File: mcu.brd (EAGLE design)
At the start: 100 x 80 mm, 62 parts, among them IC1 MCP73831/OT, T1 SI7051-A20, U12 BQ297XY, U4 NRF52832, U7 CP2102N-A01-GQFN24, X1 LFXTAL069526, X6 32.768kHz

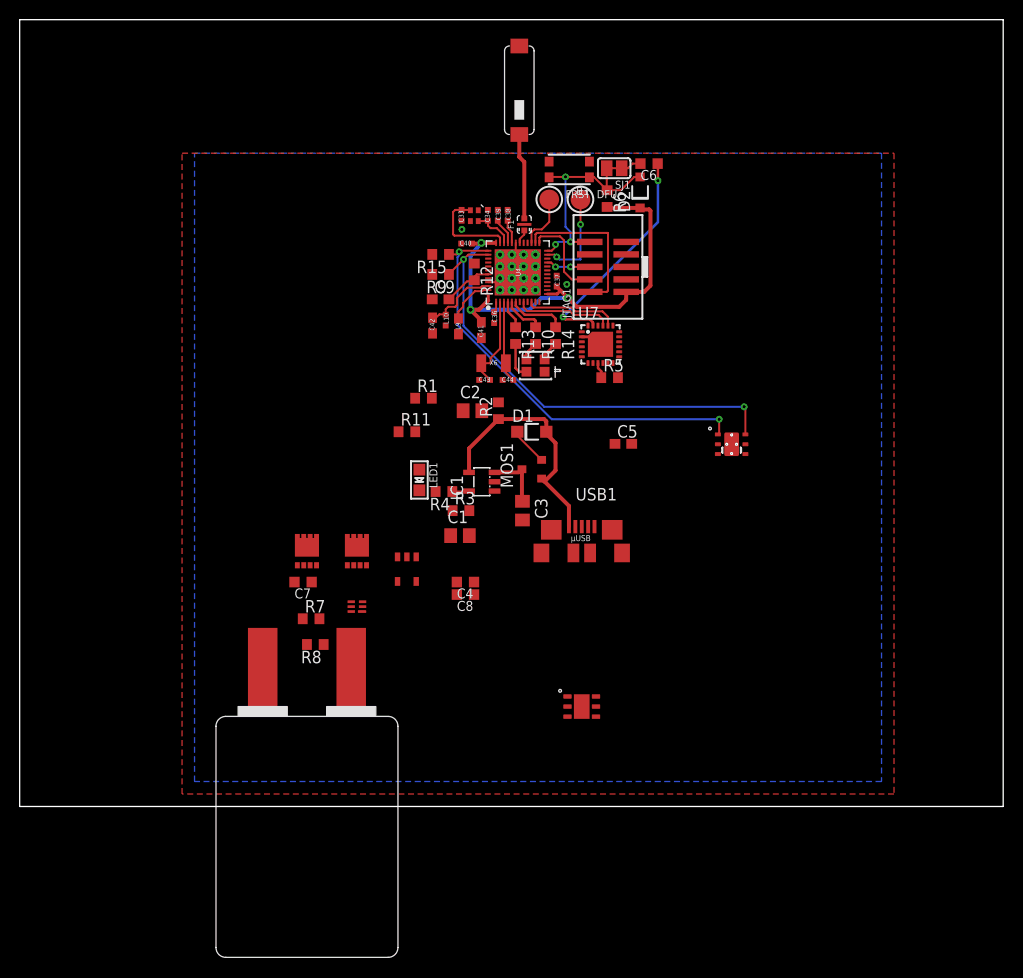
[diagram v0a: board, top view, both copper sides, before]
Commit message: UPD: finished wiring
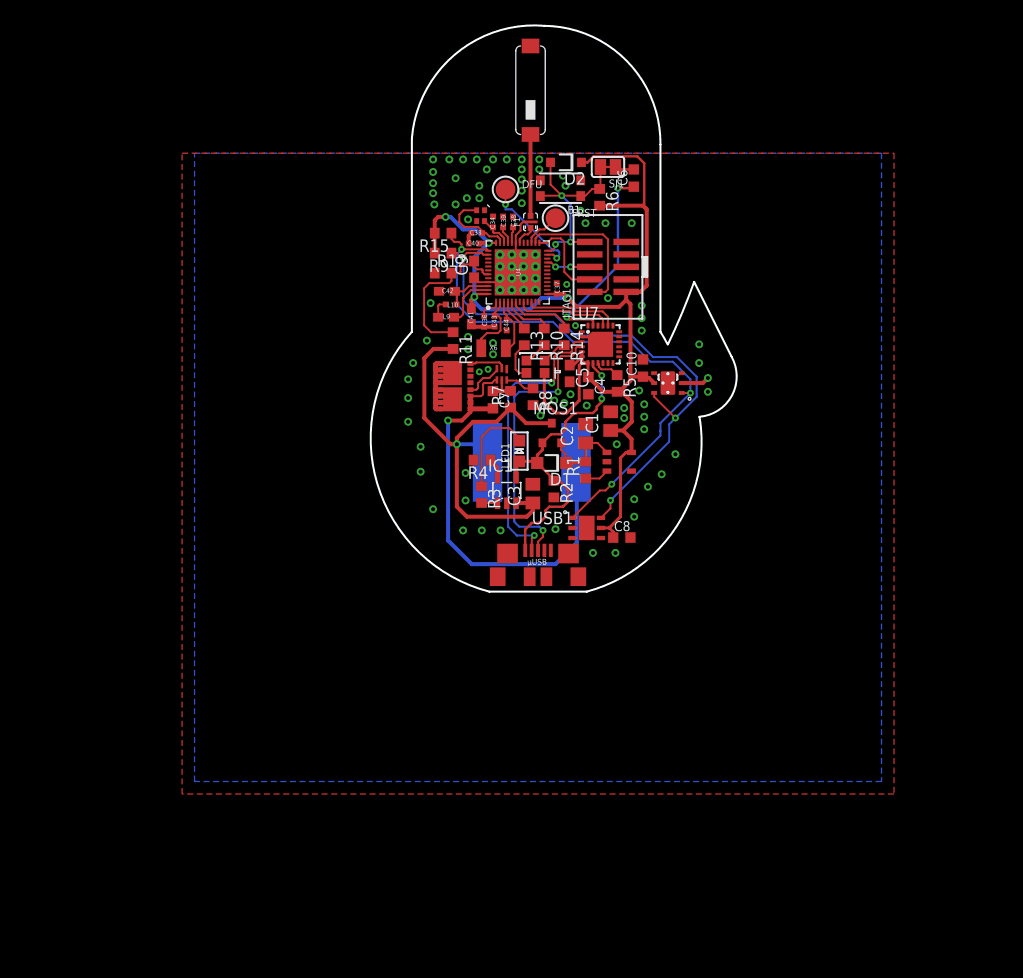
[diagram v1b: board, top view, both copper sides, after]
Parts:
- added C10: 0.1µF, rcl:C0603K
- moved U$14 36.8 mm to (52.1, 39.0), flipped to the bottom, turned to 180 degrees
- moved R8 33.5 mm to (52.2, 41.7), turned to 270 degrees
- moved R7 30.2 mm to (49.9, 41.4), turned to 90 degrees
- moved U12 27.8 mm to (49.0, 43.9), turned to 180 degrees
- moved C7 26.8 mm to (48.1, 41.4), turned to 270 degrees
- moved LDO1 24.2 mm to (61.0, 35.1), turned to 90 degrees
- moved C4 23.6 mm to (57.8, 42.8), turned to 270 degrees
- moved DSG 22.5 mm to (45.0, 41.4), turned to 90 degrees
- moved CHG 21.5 mm to (45.0, 44.1), turned to 90 degrees
- moved C1 19.2 mm to (60.1, 39.2), turned to 90 degrees
- moved T1 18.2 mm to (57.7, 28.3)
- moved R1 18.0 mm to (57.5, 34.2), turned to 90 degrees
- moved C8 16.9 mm to (61.2, 27.3), turned to 0 degrees
- moved C2 11.7 mm to (57.5, 37.9), turned to 90 degrees
- moved LED1 10.6 mm to (50.8, 36.1), turned to 0 degrees
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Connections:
- net GND: now also C10.2
- net V+: now also C10.1
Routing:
- net V+: track 50.0 -> 120.5 mm, vias 3 -> 4
- net N$16: track 0.00 -> 46.2 mm, vias 0 -> 1
- net VBAT: track 6.19 -> 47.9 mm, vias 0 -> 1
- net USBD+: track 0.00 -> 29.9 mm, vias 0 -> 2
- net USBD-: track 0.00 -> 29.4 mm, vias 0 -> 2
- net P0.25: track 43.8 -> 58.1 mm, vias 2 -> 3
- net N$11: track 0.00 -> 11.7 mm
- net P0.31: track 5.21 -> 16.5 mm
- net P0.26: track 46.4 -> 57.4 mm, vias 2 -> 3
- net GND: track 24.0 -> 34.8 mm, vias 2 -> 80
- net N$4: track 0.00 -> 9.91 mm
- net VUSB: track 24.6 -> 32.6 mm, vias 0 -> 2
- net N$2: track 3.89 -> 8.76 mm
- net N$12: track 0.00 -> 3.98 mm
- net N$14: track 0.00 -> 3.71 mm
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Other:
- board size 100 x 80 mm -> 37.2 x 57.6 mm
